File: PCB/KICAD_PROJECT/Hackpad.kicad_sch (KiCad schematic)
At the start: 23 parts, among them J1 OLED_128x64, SW1 RotaryEncoder_Switch, U1 MCU_Seeed_XIAO_RP2040

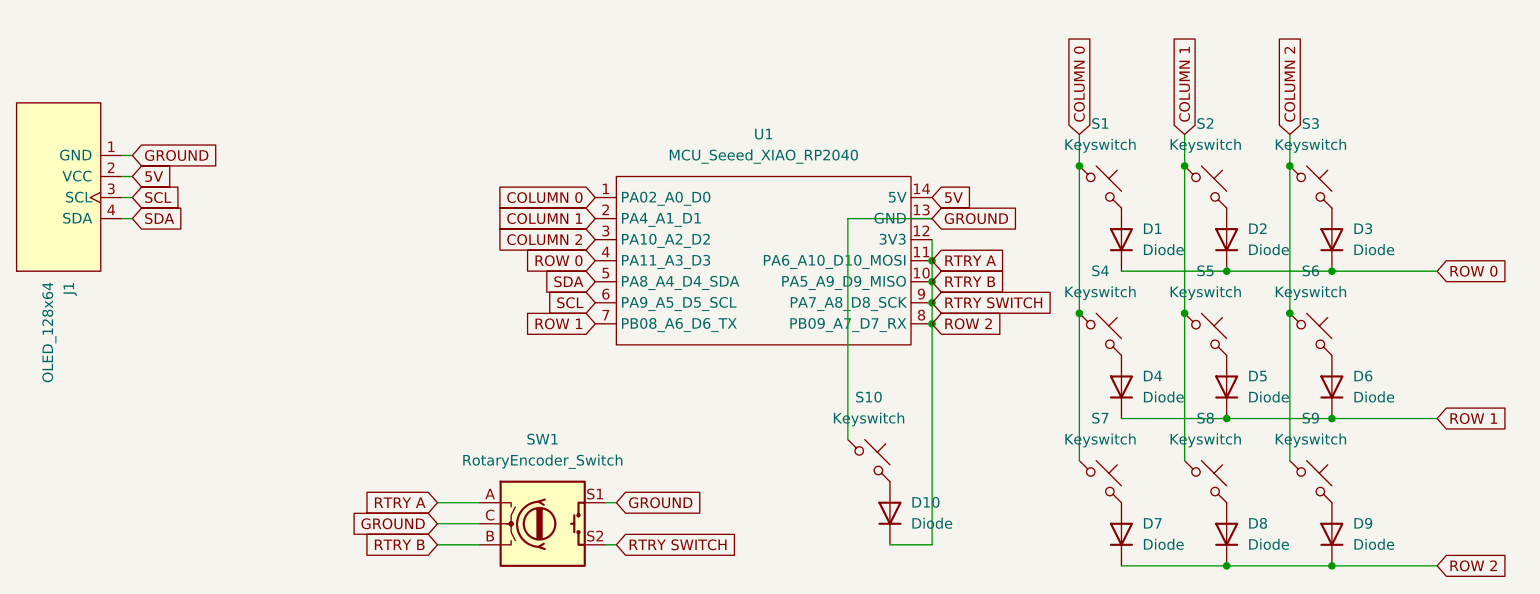
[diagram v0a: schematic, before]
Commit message: sync
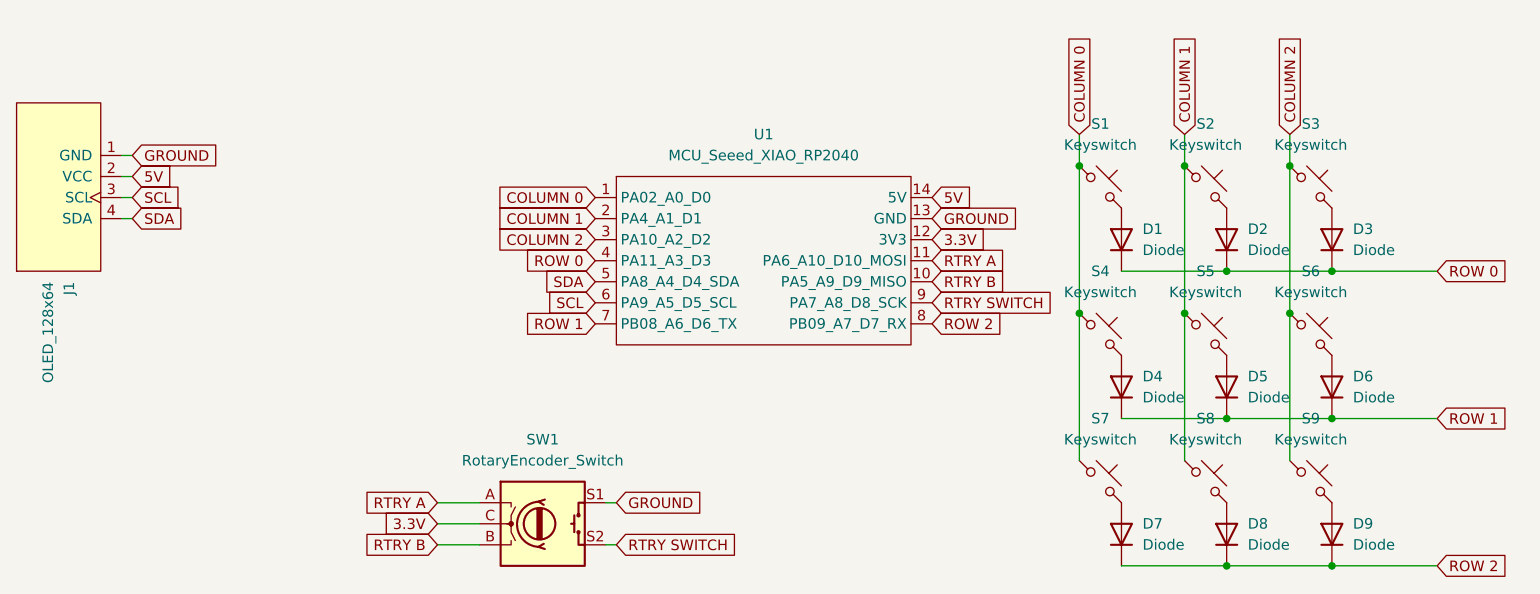
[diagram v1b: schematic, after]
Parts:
- removed D10: Diode, ScottoKeebs_Components:Diode_DO-35, symbol ScottoKeebs:Placeholder_Diode
- removed S10: Keyswitch, ScottoKeebs_Hotswap:Hotswap_MX_1.00u, symbol ScottoKeebs:Placeholder_Keyswitch
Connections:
- net GROUND: no longer SW1.C
- net ROW 2: no longer SW1.A, SW1.B, SW1.S2, U1.10 (PA5_A9_D9_MISO), U1.11 (PA6_A10_D10_MOSI), U1.12 (3V3), U1.9 (PA7_A8_D8_SCK)
- new net 3.3V: SW1.C, U1.12 (3V3)
- new net RTRY A: SW1.A, U1.11 (PA6_A10_D10_MOSI)
- new net RTRY B: SW1.B, U1.10 (PA5_A9_D9_MISO)
- new net RTRY SWITCH: SW1.S2, U1.9 (PA7_A8_D8_SCK)
